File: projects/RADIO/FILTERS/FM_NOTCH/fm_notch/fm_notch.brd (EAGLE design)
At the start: 40 x 25 mm, 20 parts

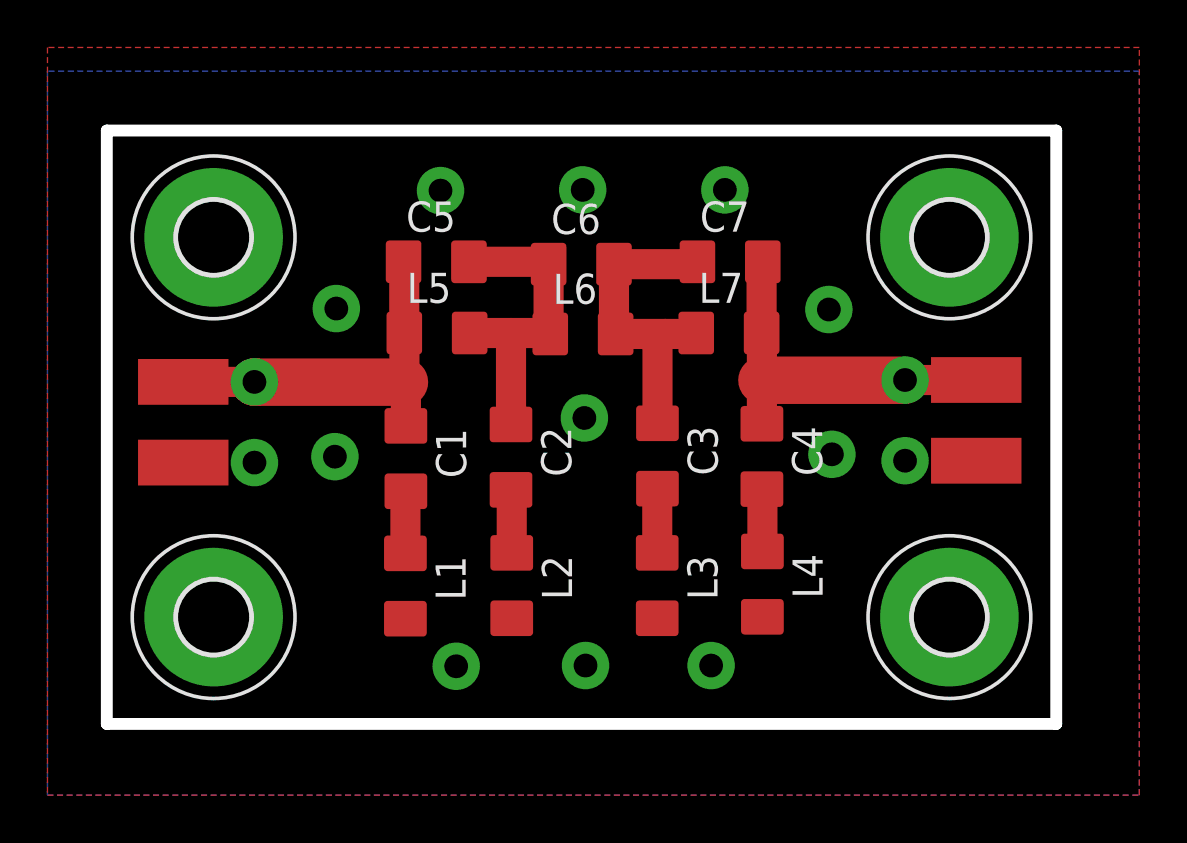
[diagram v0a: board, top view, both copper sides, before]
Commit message: update
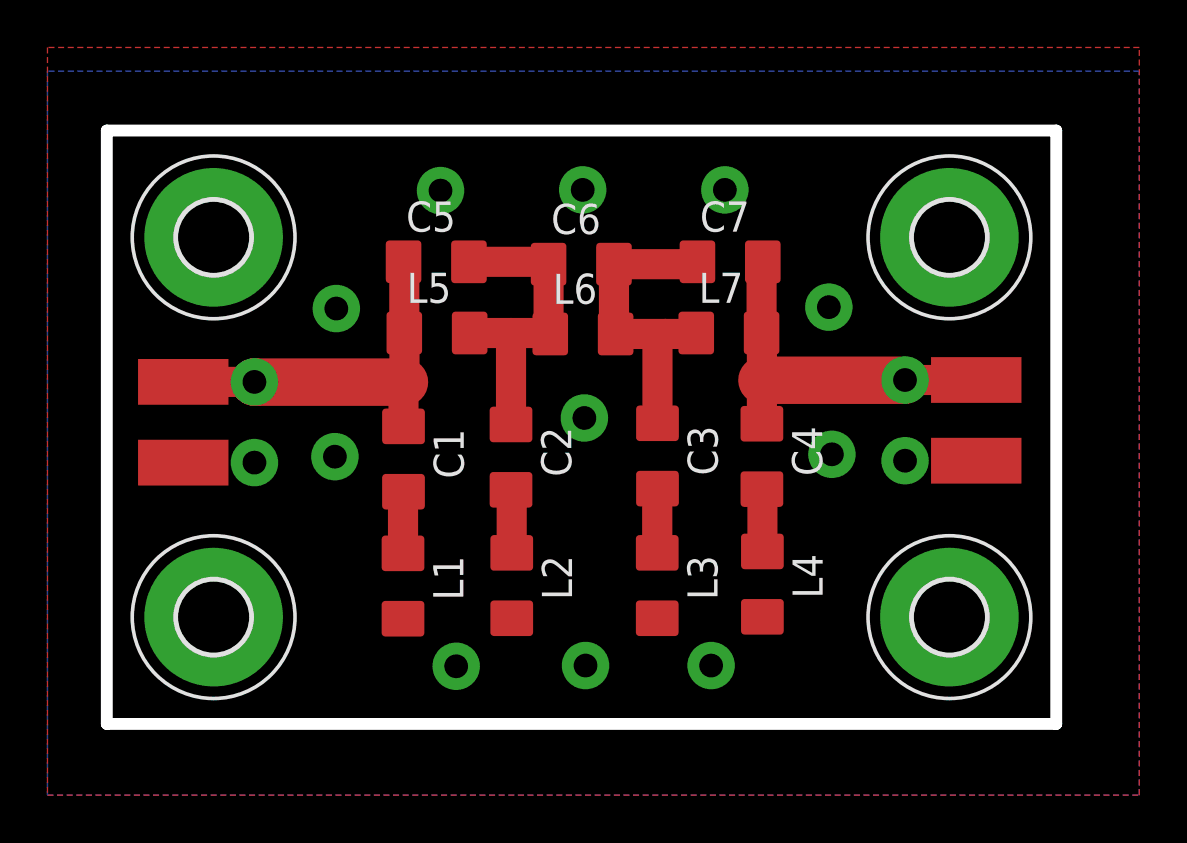
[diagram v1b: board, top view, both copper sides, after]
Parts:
- moved C1 0.10 mm to (12.5, 11.2)
- moved L1 0.10 mm to (12.5, 5.81)
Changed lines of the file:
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@@
 <wire x1="40" y1="25" x2="0" y2="25" width="0.5" layer="20" locked="yes"/>
 <wire x1="0" y1="25" x2="0" y2="0" width="0.5" layer="20" locked="yes"/>
+<dimension x1="0" y1="25" x2="0" y2="0" x3="-5" y3="12.5" textsize="1.778" layer="47"/>
+<dimension x1="0" y1="0" x2="40" y2="0" x3="20" y3="-6" textsize="1.778" layer="47"/>
 </plain>
 <attributes>
@@
 </autorouter>
 <elements>
-<element name="C1" library="mylib" package="C0805" value="8pF" x="12.6" y="11.18" smashed="yes" rot="R270">
-<attribute name="NAME" x="13.87" y="12.45" size="1.27" layer="25" rot="R270"/>
-<attribute name="VALUE" x="10.06" y="12.45" size="1.27" layer="27" rot="R270"/>
+<element name="C1" library="mylib" package="C0805" value="8pF" x="12.5" y="11.16" smashed="yes" rot="R270">
+<attribute name="NAME" x="13.77" y="12.43" size="1.27" layer="25" rot="R270"/>
+<attribute name="VALUE" x="9.96" y="12.43" size="1.27" layer="27" rot="R270"/>
 </element>
 <element name="C2" library="mylib" package="C0805" value="15pF" x="17.03" y="11.24" smashed="yes" rot="R270">
@@
 </element>
 <element name="INPUT" library="mylib" package="2X_SMD_PTH" value="INPUT" x="3.22" y="12.71" smashed="yes"/>
-<element name="L1" library="mylib" package="C0805" value="330nH" x="12.58" y="5.81" smashed="yes" rot="R270">
-<attribute name="NAME" x="13.85" y="7.08" size="1.27" layer="25" rot="R270"/>
-<attribute name="VALUE" x="10.04" y="7.08" size="1.27" layer="27" rot="R270"/>
+<element name="L1" library="mylib" package="C0805" value="330nH" x="12.48" y="5.81" smashed="yes" rot="R270">
+<attribute name="NAME" x="13.75" y="7.08" size="1.27" layer="25" rot="R270"/>
+<attribute name="VALUE" x="9.94" y="7.08" size="1.27" layer="27" rot="R270"/>
 </element>
 <element name="L2" library="mylib" package="C0805" value="180nH" x="17.06" y="5.83" smashed="yes" rot="R270">
@@
 <contactref element="INPUT" pad="P$1"/>
 <wire x1="3.22" y1="14.41" x2="6.22" y2="14.41" width="1.27" layer="1"/>
-<wire x1="12.54" y1="14.4" x2="6.23" y2="14.4" width="2" layer="1"/>
+<wire x1="6.23" y1="14.4" x2="12.54" y2="14.4" width="2" layer="1"/>
 <wire x1="6.22" y1="14.41" x2="6.23" y2="14.4" width="2" layer="1"/>
-<wire x1="12.54" y1="13.96" x2="12.54" y2="14.4" width="1.27" layer="1"/>
-<wire x1="12.54" y1="14.46" x2="12.54" y2="16.463" width="1.27" layer="1"/>
 <wire x1="12.54" y1="16.463" x2="12.533" y2="16.47" width="1.27" layer="1"/>
 <wire x1="12.533" y1="16.47" x2="12.533" y2="19.44" width="1.27" layer="1"/>
 <wire x1="12.533" y1="19.44" x2="12.503" y2="19.47" width="1.27" layer="1"/>
-<wire x1="12.6" y1="12.557" x2="12.6" y2="13.9" width="1.27" layer="1"/>
-<wire x1="12.6" y1="13.9" x2="12.54" y2="13.96" width="1.27" layer="1"/>
-<wire x1="12.6" y1="12.557" x2="12.54" y2="14.46" width="0" layer="19" extent="1-1"/>
+<wire x1="12.5" y1="12.537" x2="12.5" y2="14.36" width="1.27" layer="1"/>
+<wire x1="12.5" y1="14.36" x2="12.54" y2="14.4" width="1.27" layer="1"/>
+<wire x1="12.54" y1="14.4" x2="12.54" y2="16.463" width="1.27" layer="1"/>
+<wire x1="12.54" y1="16.463" x2="12.533" y2="16.47" width="1.27" layer="1"/>
 </signal>
 <signal name="N$4">
@@
 <contactref element="L1" pad="1"/>
 <contactref element="C1" pad="2"/>
-<wire x1="12.58" y1="7.187" x2="12.58" y2="9.783" width="1.27" layer="1"/>
-<wire x1="12.58" y1="9.783" x2="12.6" y2="9.803" width="1.27" layer="1"/>
+<wire x1="12.48" y1="9.763" x2="12.48" y2="7.187" width="1.27" layer="1"/>
+<wire x1="12.5" y1="9.783" x2="12.48" y2="9.763" width="1.27" layer="1"/>
 </signal>
 <signal name="N$3">
@@
 <via x="20.12" y="12.89" extent="1-16" drill="1" diameter="2" shape="octagon"/>
 <via x="9.67" y="17.5" extent="1-16" drill="1" diameter="2" shape="octagon"/>
-<via x="30.42" y="17.46" extent="1-16" drill="1" diameter="2" shape="octagon"/>
+<via x="30.42" y="17.56" extent="1-16" drill="1" diameter="2" shape="octagon"/>
 </signal>
 <signal name="N$8">
